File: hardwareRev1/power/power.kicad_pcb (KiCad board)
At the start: 2 copper layers, 34.2 x 24.7 mm, 28 parts, among them IC1 ATTINY24A-M-FIXED, P1 VIN, P2 CONN_11X2, P3 AVRProg, U1 TPS63020, U2 NCP508

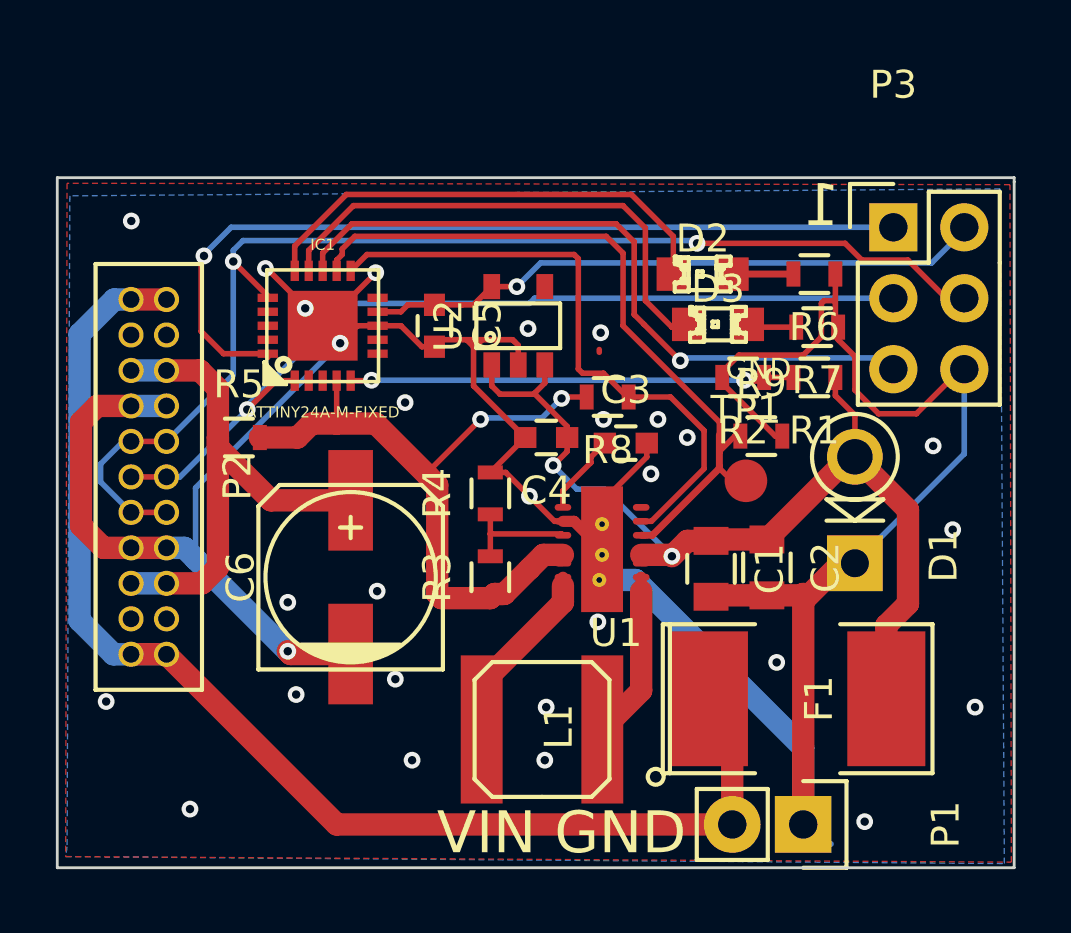
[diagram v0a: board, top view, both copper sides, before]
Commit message: board is almost done. Commiting before I destroy all my work...
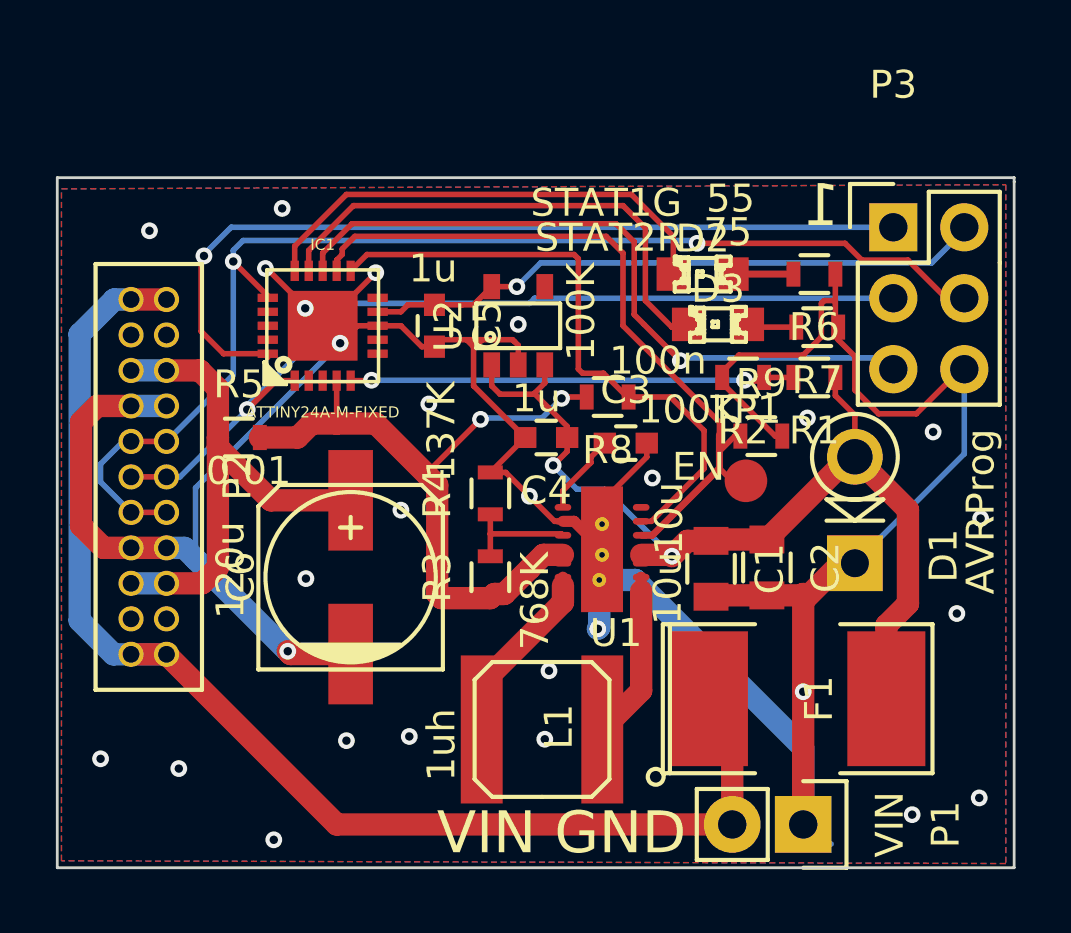
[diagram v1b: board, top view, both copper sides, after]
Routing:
- net GND: track 115.4 -> 117.5 mm, vias 26 -> 17
- net (no net): track 0.10 -> 0.27 mm, vias 3 -> 11
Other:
- board text removed: "GND"
